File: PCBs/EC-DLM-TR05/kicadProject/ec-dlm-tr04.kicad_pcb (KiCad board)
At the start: 2 copper layers, 28 x 53 mm, 23 parts, among them J1 input, J2 LED Connector, J3 RJ45, U1 MCP6424, U2 LD1117S50TR

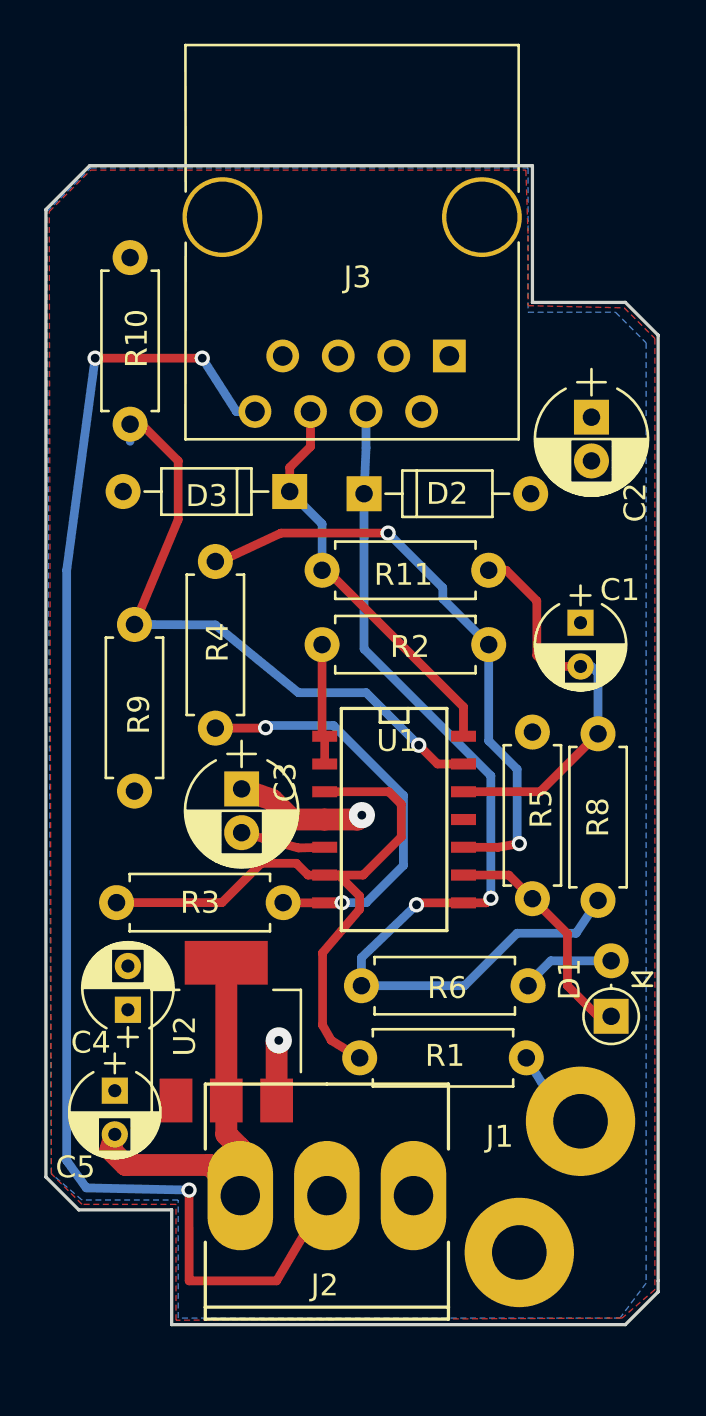
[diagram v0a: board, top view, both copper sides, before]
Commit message: Revision board rev9
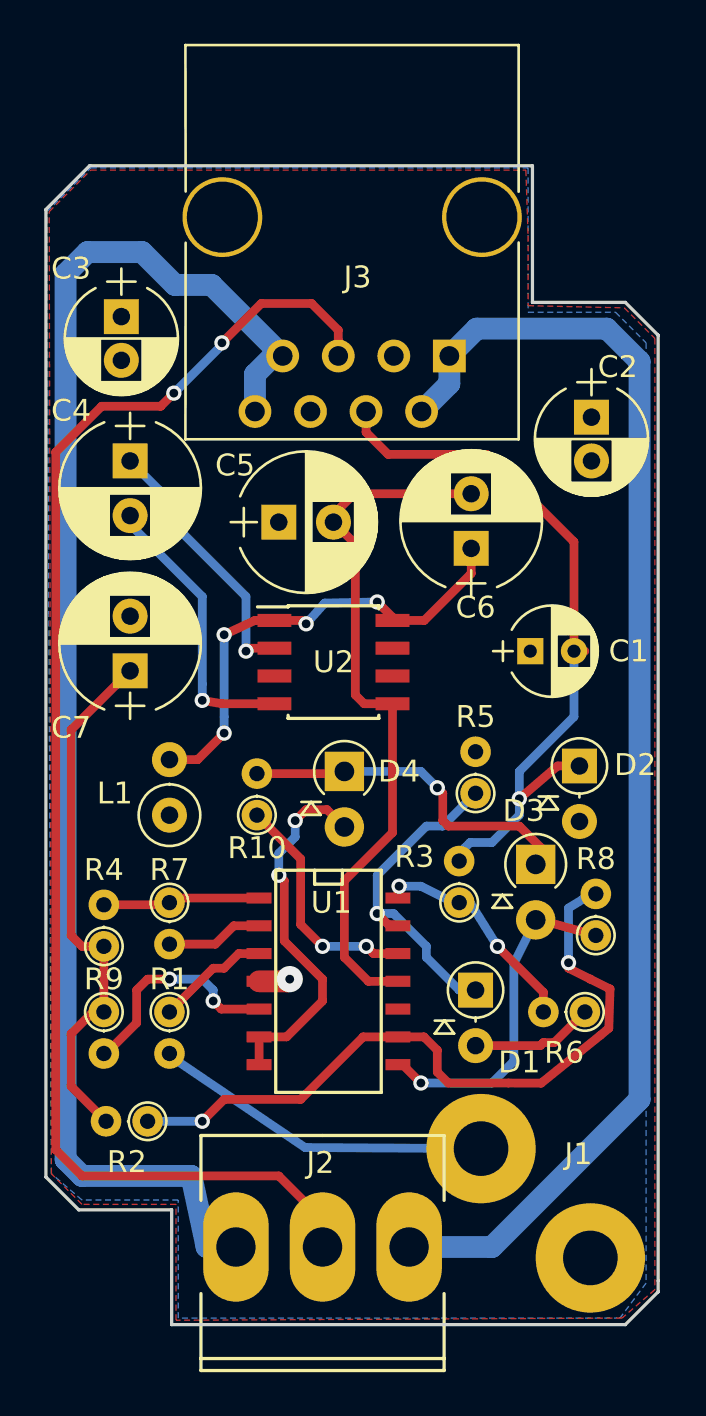
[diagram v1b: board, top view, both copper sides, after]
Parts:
- removed R11: 470k, Resistors_THT:R_Axial_DIN0207_L6.3mm_D2.5mm_P7.62mm_Horizontal
- added C6: 100u, Capacitors_THT:CP_Radial_D6.3mm_P2.50mm, F.Cu at (158.6, 86.6)
- added C7: 104, Capacitors_THT:CP_Radial_D6.3mm_P2.50mm, F.Cu at (143.0, 92.2)
- added D4: D, Diodes_THT:D_A-405_P2.54mm_Vertical_AnodeUp, F.Cu at (152.8, 96.8)
- added L1: Ferrite_Bead, Inductors_THT:L_Axial_L6.6mm_D2.7mm_P2.54mm_Vertical_Vishay_IM-2, F.Cu at (144.8, 98.8)
- added R7: 10k, Resistors_THT:R_Axial_DIN0204_L3.6mm_D1.6mm_P1.90mm_Vertical, F.Cu at (144.8, 102.8)
- C1: value 104 -> 105
- C4: value 105 -> 10u; footprint Capacitors_THT:CP_Radial_D4.0mm_P2.00mm -> Capacitors_THT:CP_Radial_D6.3mm_P2.50mm
- C5: value 4.7pF -> 10u; footprint Capacitors_THT:CP_Radial_D4.0mm_P2.00mm -> Capacitors_THT:CP_Radial_D6.3mm_P2.50mm
- D2: value BZX79C3V3 -> BZX79C5V; footprint Diodes_THT:D_DO-35_SOD27_P7.62mm_Horizontal -> Diodes_THT:D_DO-35_SOD27_P2.54mm_Vertical_AnodeUp
- D3: value BZX79C3V3‎ -> D; footprint Diodes_THT:D_DO-35_SOD27_P7.62mm_Horizontal -> Diodes_THT:D_A-405_P2.54mm_Vertical_AnodeUp
- R1: value 27k -> 100k; footprint Resistors_THT:R_Axial_DIN0207_L6.3mm_D2.5mm_P7.62mm_Horizontal -> Resistors_THT:R_Axial_DIN0204_L3.6mm_D1.6mm_P1.90mm_Vertical
- R10: value 33k -> 10k; footprint Resistors_THT:R_Axial_DIN0207_L6.3mm_D2.5mm_P7.62mm_Horizontal -> Resistors_THT:R_Axial_DIN0204_L3.6mm_D1.6mm_P1.90mm_Vertical
- R2: value 7.5k -> 10k; footprint Resistors_THT:R_Axial_DIN0207_L6.3mm_D2.5mm_P7.62mm_Horizontal -> Resistors_THT:R_Axial_DIN0204_L3.6mm_D1.6mm_P1.90mm_Vertical
- R3, R4, R5, R6, R8: footprint Resistors_THT:R_Axial_DIN0207_L6.3mm_D2.5mm_P7.62mm_Horizontal -> Resistors_THT:R_Axial_DIN0204_L3.6mm_D1.6mm_P1.90mm_Vertical
- R9: value 470k -> 10k; footprint Resistors_THT:R_Axial_DIN0207_L6.3mm_D2.5mm_P7.62mm_Horizontal -> Resistors_THT:R_Axial_DIN0204_L3.6mm_D1.6mm_P1.90mm_Vertical
- U1: value MCP6424 -> TL074
- U2: value LD1117S50TR -> TC1044S; footprint TO_SOT_Packages_SMD:SOT-223 -> Housings_SOIC:SOIC-8_3.9x4.9mm_Pitch1.27mm
- moved C5 27.1 mm to (149.8, 85.4), turned to 0 degrees
- moved R2 26.8 mm to (143.8, 112.8)
- moved R10 26.2 mm to (148.8, 98.8), turned to 90 degrees
- moved C4 25.1 mm to (143.0, 82.6), turned to 270 degrees
- moved C3 22.3 mm to (142.6, 76.0)
- moved D3 20.4 mm to (161.6, 101.0), turned to 270 degrees
- moved R4 18.3 mm to (141.8, 104.8), turned to 90 degrees
- moved U2 17.6 mm to (152.3, 91.8), turned to 0 degrees
- moved D2 15.9 mm to (163.6, 96.5), turned to 270 degrees
- moved R9 10.2 mm to (141.8, 107.8), turned to 270 degrees
- moved R1 8.95 mm to (144.8, 107.8), turned to 270 degrees
- moved R3 8.05 mm to (158.1, 102.8), turned to 90 degrees
- moved U1 7.98 mm to (152.2, 106.4)
- moved D1 6.32 mm to (158.8, 106.8), turned to 270 degrees
- moved R5 3.82 mm to (158.8, 97.8), turned to 90 degrees
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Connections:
- C1 pad 1: GND -> AGND
- C1 pad 2: Net-(C1-Pad2) -> ADCTrig
- C2 pad 1: VCC5 -> AVCC
- C2 pad 2: GND -> AGND
- C3 pad 1: VCC5 -> AVCC
- C3 pad 2: GND -> AGND
- C4 pad 1: GND -> Net-(C4-Pad1)
- C4 pad 2: VCC5 -> Net-(C4-Pad2)
- C5 pad 1: GND -> AGND
- C5 pad 2: VCC5-LDO -> AVSS
- D2 pad 1: ADCInput -> ADCTrig
- D2 pad 2: GND -> AGND
- D3 pad 1: SchmidtTrigInput -> Net-(D3-Pad1)
- D3 pad 2: GND -> Net-(D3-Pad2)
- J1 pad 1: GND -> AGND
- J2 pad 2: WSLED-Signal -> L_OUT_5
- J2 pad 3: VCC5-LDO -> VCC5
- J3 pad 2: (no net) -> GND
- J3 pad 3: GND -> AGND
- J3 pad 4: ADCInput -> ADCTrig
- J3 pad 5: VCC5 -> L_OUT_5
- J3 pad 6: SchmidtTrigInput -> AVCC
- J3 pad 8: WSLED-Signal -> VCC5
- R10 pad 1: GND -> Net-(R10-Pad1)
- R10 pad 2: Net-(R10-Pad2) -> Net-(D3-Pad1)
- R2 pad 2: Net-(R2-Pad2) -> Net-(C7-Pad1)
- R3 pad 2: Net-(R1-Pad1) -> ADCTrig
- R4 pad 1: Net-(R2-Pad1) -> Net-(C7-Pad1)
- R4 pad 2: Net-(R3-Pad1) -> Net-(R4-Pad2)
- R5 pad 1: GND -> Net-(D1-Pad1)
- R5 pad 2: Net-(D1-Pad1) -> AGND
- R6 pad 2: ADCInput -> Net-(R3-Pad1)
- R8 pad 1: ADCInput -> Net-(D3-Pad2)
- R8 pad 2: Net-(C1-Pad2) -> Net-(R2-Pad1)
- R9 pad 1: VCC5 -> Net-(C7-Pad1)
- R9 pad 2: Net-(R10-Pad2) -> Net-(R9-Pad2)
- U1 pad 1: Net-(R2-Pad2) -> Net-(R4-Pad2)
- U1 pad 10: Net-(R2-Pad1) -> AGND
- U1 pad 11: GND -> AVSS
- U1 pad 12: Net-(C1-Pad2) -> Net-(R10-Pad1)
- U1 pad 13: Net-(R10-Pad2) -> Net-(D1-Pad1)
- U1 pad 14: SchmidtTrigInput -> Net-(R3-Pad1)
- U1 pad 2: Net-(R2-Pad2) -> Net-(R7-Pad2)
- U1 pad 4: VCC5 -> AVCC
- U1 pad 5: GND -> Net-(R9-Pad2)
- U1 pad 6: Net-(R1-Pad1) -> Net-(D4-Pad2)
- U1 pad 7: Net-(R3-Pad1) -> Net-(D4-Pad2)
- U1 pad 8: ADCInput -> Net-(D3-Pad2)
- U1 pad 9: Net-(D1-Pad1) -> Net-(R2-Pad1)
- U2 pad 1: GND -> Net-(C6-Pad1)
- U2 pad 2: VCC5-LDO -> Net-(C4-Pad1)
- U2 pad 3: VCC5 -> AGND
- U2 pad 4: VCC5-LDO -> Net-(C4-Pad2)
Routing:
- net L_OUT_5: track 0.00 -> 65.9 mm, vias 0 -> 2
- net WSLED-Signal: track 64.4 -> 0.00 mm, vias 3 -> 0
- net VCC5: track 8.83 -> 66.9 mm, vias 2 -> 0
- net GND: track 3.89 -> 60.0 mm
- net ADCInput: track 45.6 -> 0.00 mm, vias 2 -> 0
- net ADCTrig: track 0.00 -> 34.3 mm, vias 0 -> 1
- net AVSS: track 0.00 -> 32.6 mm
- net Net-(R10-Pad2): track 29.1 -> 0.00 mm, vias 1 -> 0
- net Net-(R1-Pad1): track 30.8 -> 5.20 mm
- net Net-(C7-Pad1): track 0.00 -> 24.5 mm
- net Net-(C6-Pad1): track 0.00 -> 21.9 mm, vias 0 -> 4
- net SchmidtTrigInput: track 18.7 -> 0.00 mm
- net VCC5-LDO: track 18.5 -> 0.00 mm
- net Net-(C1-Pad2): track 18.4 -> 0.00 mm
- net Net-(D4-Pad2): track 0.00 -> 17.0 mm, vias 0 -> 2
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- added copper zone on F.Cu, net AGND
- added copper zone on B.Cu, net AVCC
- removed copper zone on F.Cu, net GND
- removed copper zone on B.Cu, net VCC5
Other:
- board text added: "TR07 - Litioo - 2019"
- board text removed: "TR06 - Litioo - 2018"
